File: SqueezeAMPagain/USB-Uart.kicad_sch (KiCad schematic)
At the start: 21 parts, among them J7 USB_B_Micro, Q4 Q_NPN_BEC, Q5 Q_NPN_BEC, U6 CP2102N-Axx-xQFN28

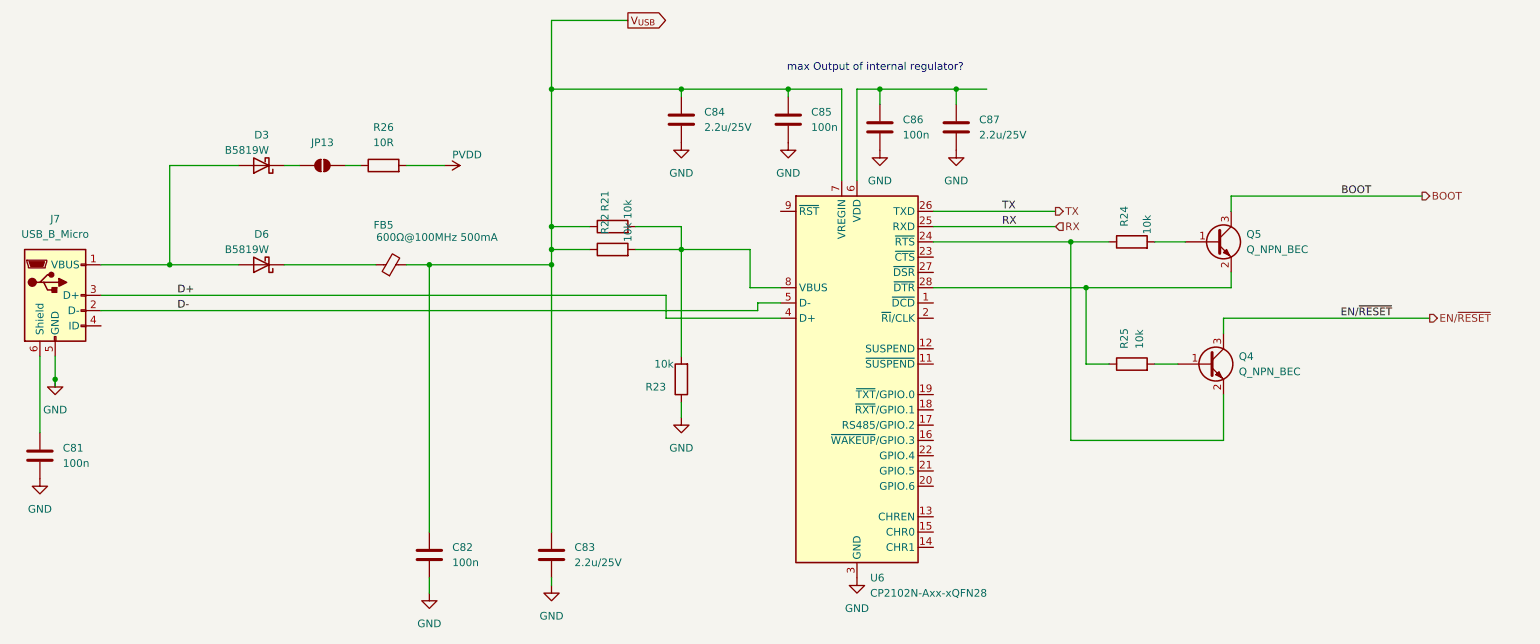
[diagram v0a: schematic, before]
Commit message: v2
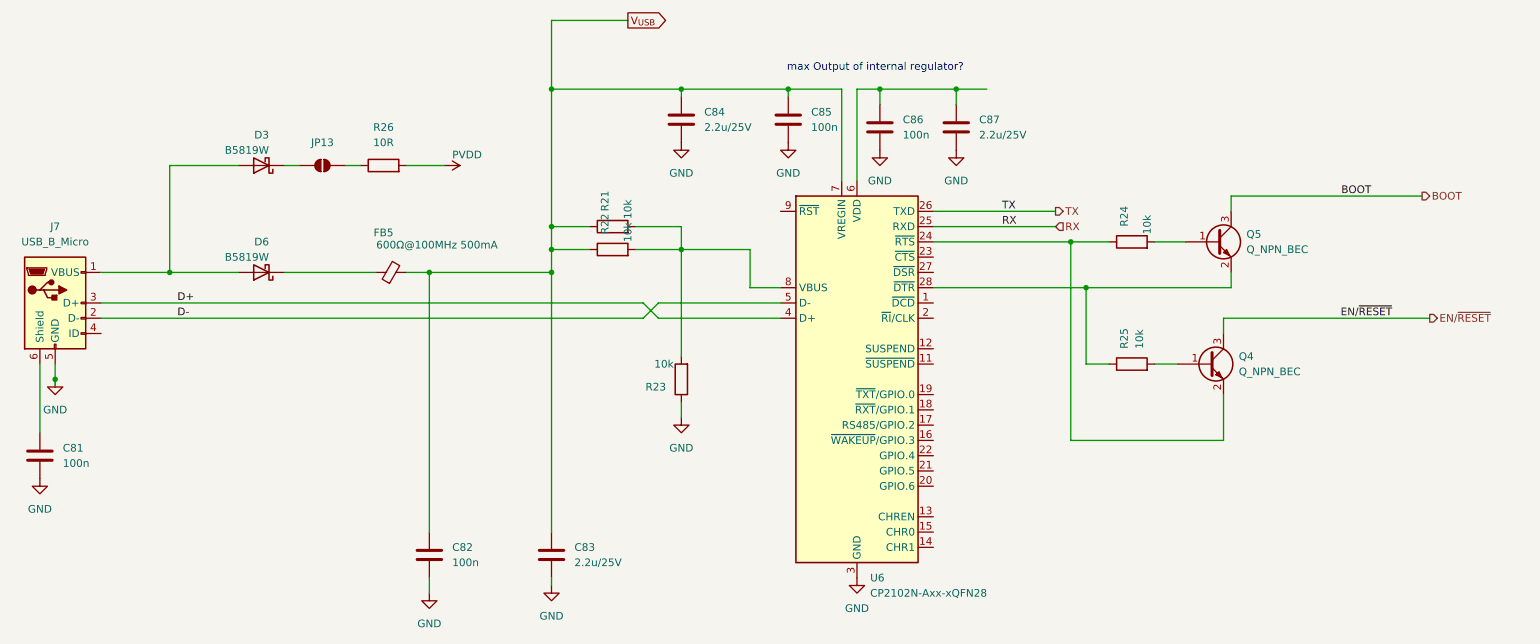
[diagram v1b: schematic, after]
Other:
- moved on the sheet: D6, FB5, J7
